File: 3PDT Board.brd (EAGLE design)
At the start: 23.8 x 22.2 mm, 10 parts, among them SW2 3PDT

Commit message: Fixed ground connections so jack grounds actually connect to ground!
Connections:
- net GND: now also JIG.1, JOG.1
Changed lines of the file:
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@@
 </polygon>
 <contactref element="SW2" pad="B2"/>
+<contactref element="JOG" pad="1"/>
+<contactref element="JIG" pad="1"/>
 </signal>
 <signal name="IN">

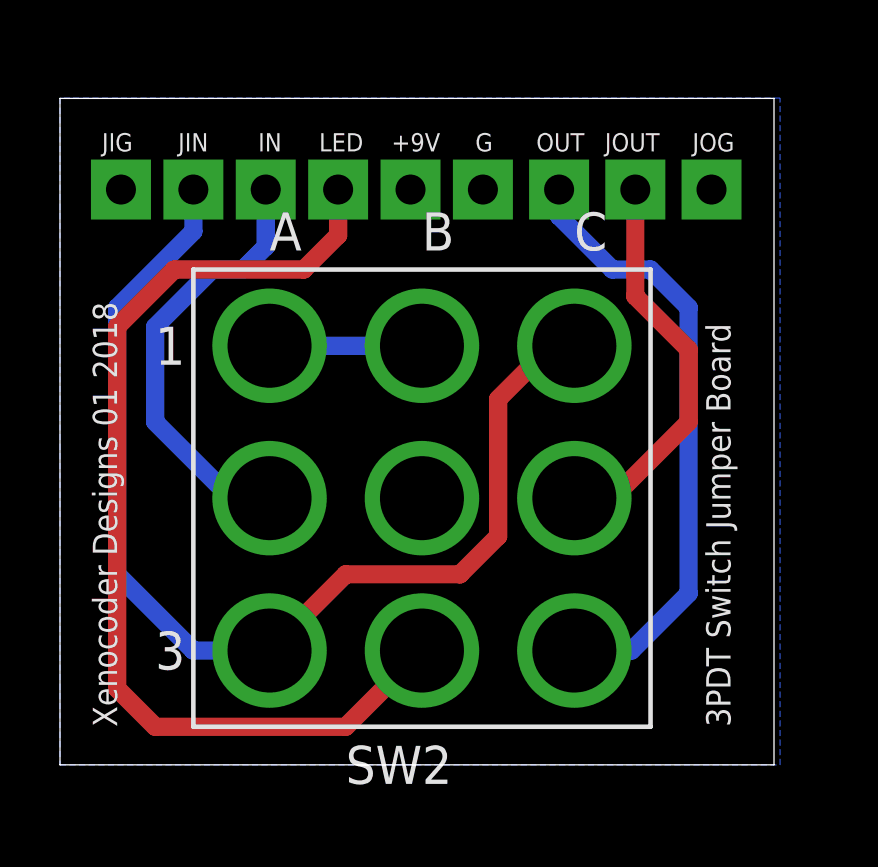
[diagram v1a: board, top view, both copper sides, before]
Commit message: Fixed circuit and made panel
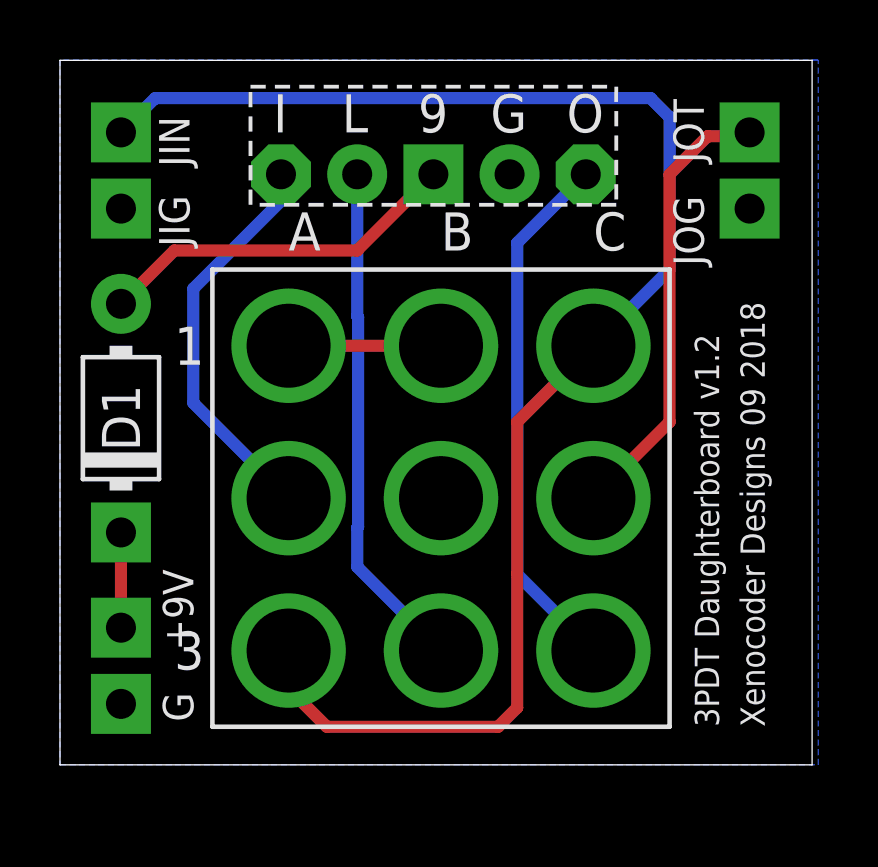
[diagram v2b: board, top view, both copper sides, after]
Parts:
- removed IN: IN(T), mb_supply:SQUARE
- removed JOUT, LED: (no value), mb_supply:SQUARE
- removed OUT: OUT(T), mb_supply:SQUARE
- added D1: 1N4001, mb_diodes:DO41-3
- added JOT: (no value), mb_supply:SQUARE
- added U$1: BOARDLINK, xc_library:BOARDLINK
- moved G 21.0 mm to (2.03, 2.03)
- moved +9V 17.5 mm to (2.03, 4.57)
- moved JIN 3.07 mm to (2.03, 21.1)
- moved JOG 1.42 mm to (23.0, 18.5)
- moved SW2 0.63 mm to (12.7, 8.89)
- moved JIG 0.63 mm to (2.03, 18.5)
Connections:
- removed net IN: IN.1, SW2.A2
- removed net OUT: OUT.1, SW2.C3
- new net +9V: +9V.1, D1.C
- new net N$5: SW2.A2, U$1.1
- new net N$6: SW2.C3, U$1.5
- new net N$7: D1.A, U$1.3
- net GND: now also U$1.4
- net N$1: now also U$1.2; no longer LED.1
- net N$2: now also JOT.1; no longer JOUT.1
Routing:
- net OUT: track 20.6 -> 0.00 mm
- net N$6: track 0.00 -> 17.9 mm
- net N$1: track 34.0 -> 17.1 mm
- net IN: track 14.7 -> 0.00 mm
- net N$4: track 37.1 -> 50.5 mm
- net N$5: track 0.00 -> 13.3 mm
- net N$7: track 0.00 -> 12.2 mm
- net +9V: track 0.00 -> 3.17 mm
- net N$2: track 13.3 -> 15.1 mm
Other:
- board size 23.8 x 22.2 mm -> 25.1 x 23.5 mm
- board text added: "3PDT Daughterboard v1.2"
- board text added: "Xenocoder Designs 09 2018"
- board text removed: "3PDT Switch Jumper Board"
- board text removed: "Xenocoder Designs 01 2018"
